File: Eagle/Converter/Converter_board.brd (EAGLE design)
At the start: 28.9 x 39.6 mm, 12 parts

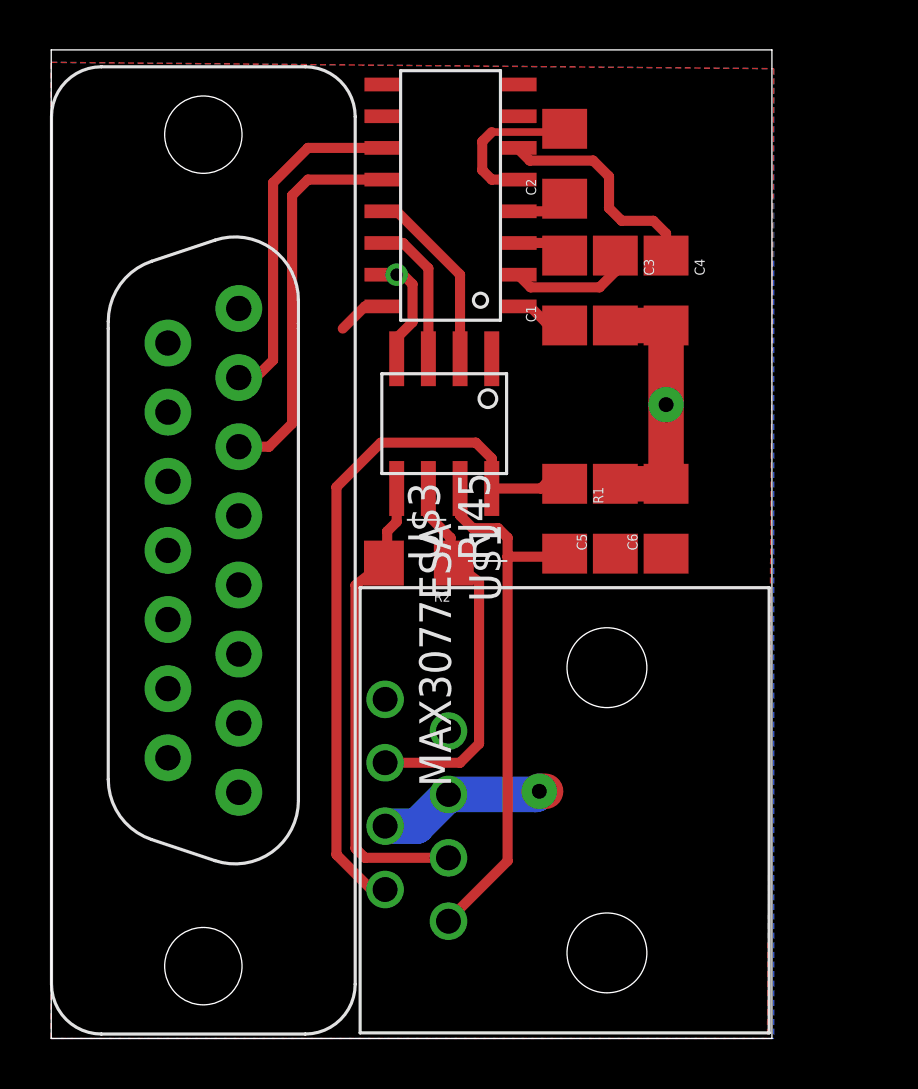
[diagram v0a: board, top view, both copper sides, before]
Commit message: rerouted board
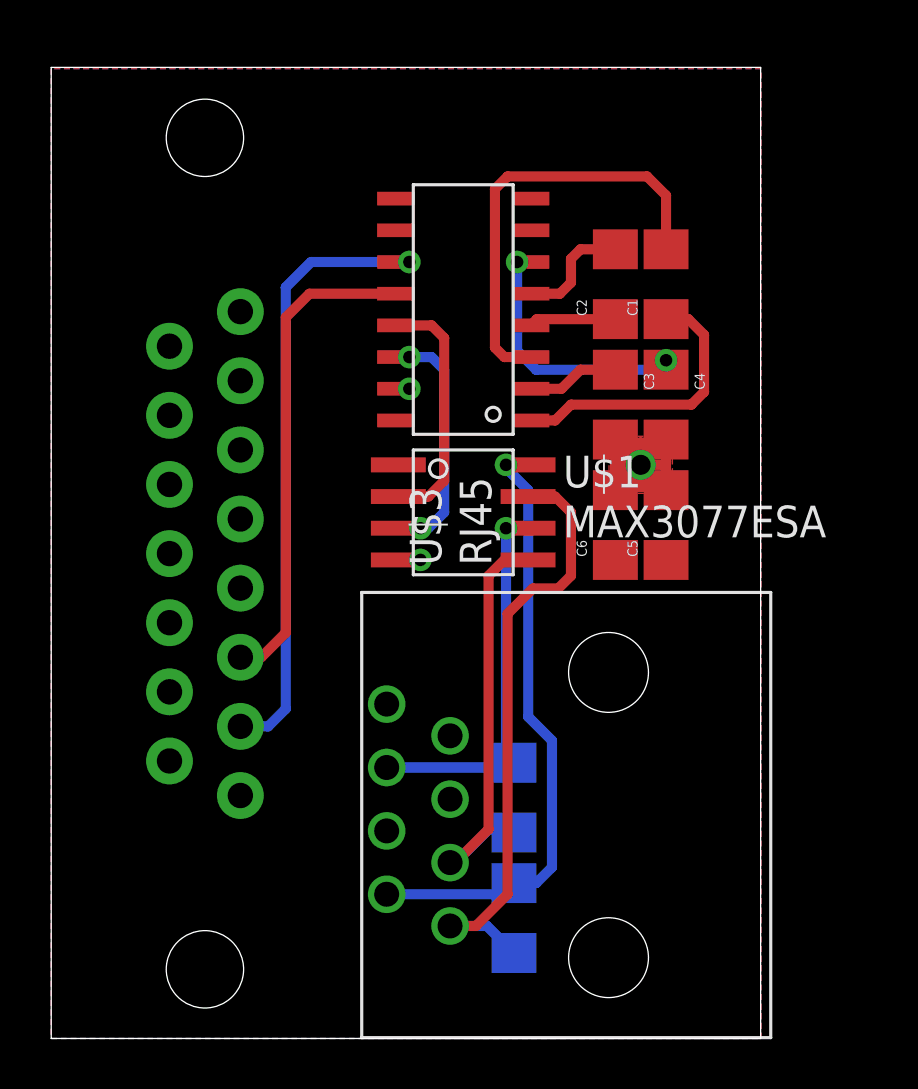
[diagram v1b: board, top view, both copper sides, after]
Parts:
- moved R1 16.1 mm to (18.5, 4.83), flipped to the bottom
- moved R2 10.1 mm to (18.5, 9.65), flipped to the bottom, turned to 270 degrees
- moved C2 5.24 mm to (22.6, 30.2)
- moved U$2 4.60 mm to (16.5, 29.2)
- moved C3 4.57 mm to (22.6, 25.4)
- moved C4 4.57 mm to (24.6, 25.4)
- moved C1 4.07 mm to (24.6, 30.2)
- moved U$1 3.64 mm to (16.5, 21.1), turned to 0 degrees
- moved C5 2.05 mm to (24.6, 20.6)
- moved C6 2.05 mm to (22.6, 20.6)
- moved U$3 0.20 mm to (20.6, 8.95)
- moved U$4 0.14 mm to (6.16, 19.4), flipped to the bottom, turned to 90 degrees
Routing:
- net N$1: track 2.08 -> 17.5 mm
- net T_IN1: track 13.8 -> 24.9 mm, vias 0 -> 1
- net N$2: track 2.19 -> 11.5 mm
- net VCC: track 9.00 -> 0.00 mm, vias 1 -> 0
- net T_OUT1: track 5.85 -> 9.96 mm, vias 0 -> 2
- net R_OUT1: track 15.6 -> 19.7 mm
- net TRANS-: track 28.7 -> 24.8 mm, vias 0 -> 1
- net TRANS+: track 22.0 -> 24.8 mm
- net R_IN1: track 7.50 -> 9.96 mm
- net N$5: track 9.01 -> 11.0 mm, vias 0 -> 2
- net REC+: track 19.1 -> 17.3 mm
- net N$4: track 6.24 -> 4.69 mm
- net N$6: track 5.24 -> 3.71 mm
- net N$3: track 2.08 -> 3.50 mm
- net GND: track 15.0 -> 14.3 mm, vias 2 -> 3
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- added copper zone on layer 1, net GND
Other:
- board size 28.9 x 39.6 mm -> 28.4 x 38.9 mm
